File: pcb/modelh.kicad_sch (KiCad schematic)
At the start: 15 parts, among them J1 Battery Conn, J2 Conn_01x16, J3 Conn_01x12, J4 Conn_01x04, U1 nice_nano, U2 74HC595, U3 74HC595

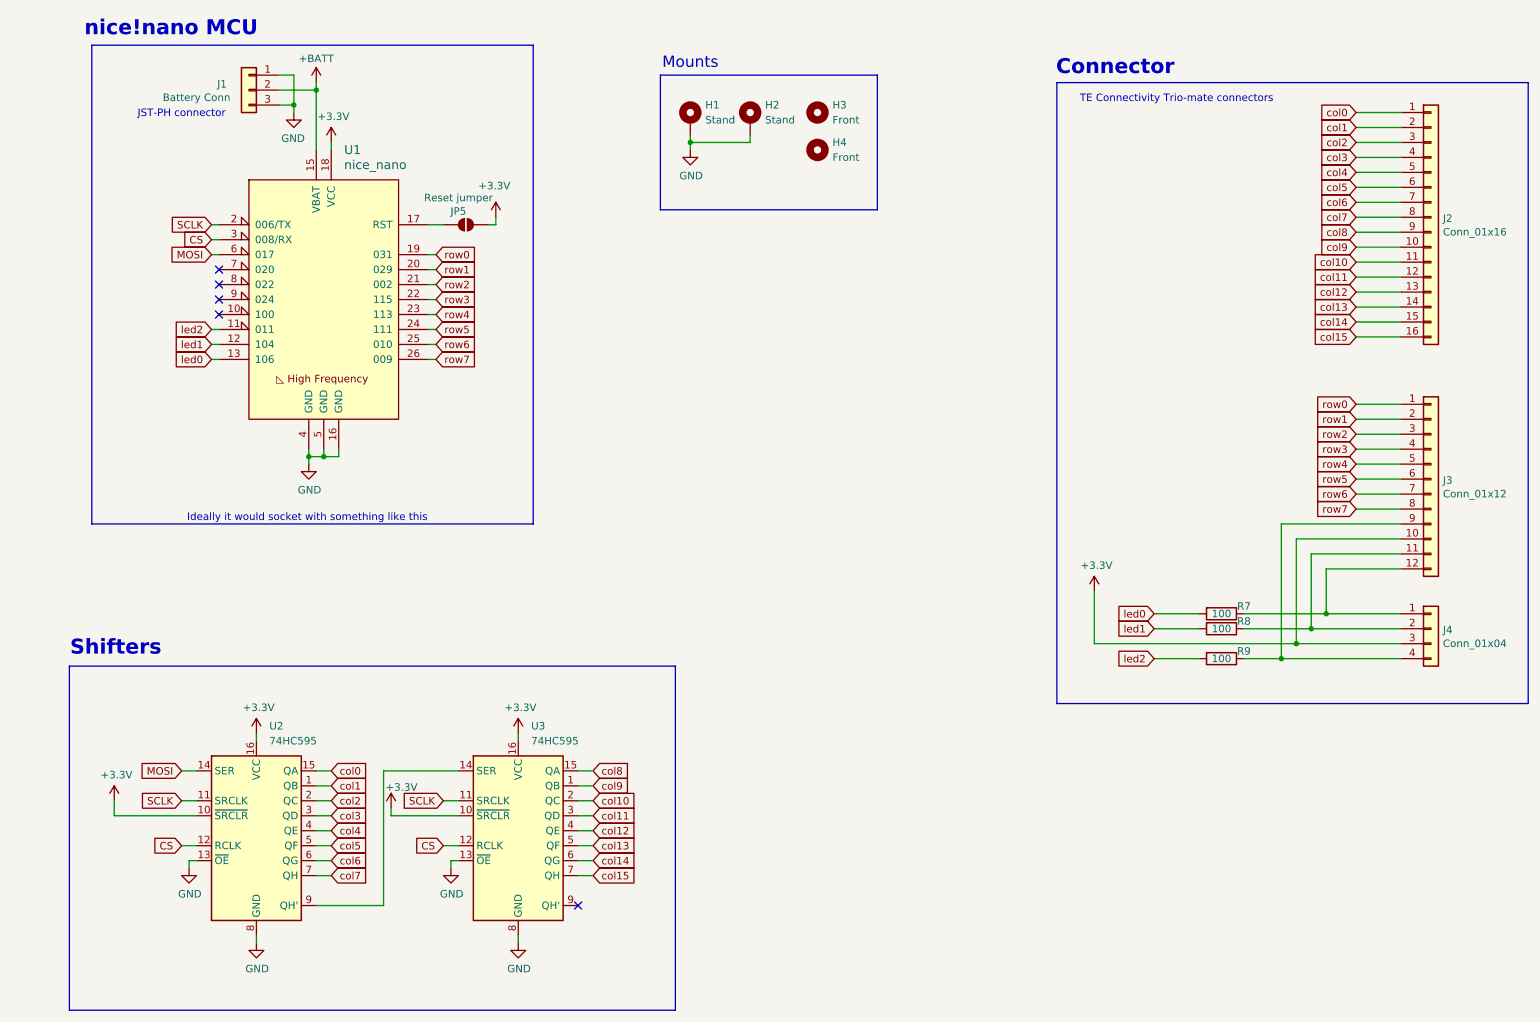
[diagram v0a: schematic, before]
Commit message: version 0.2
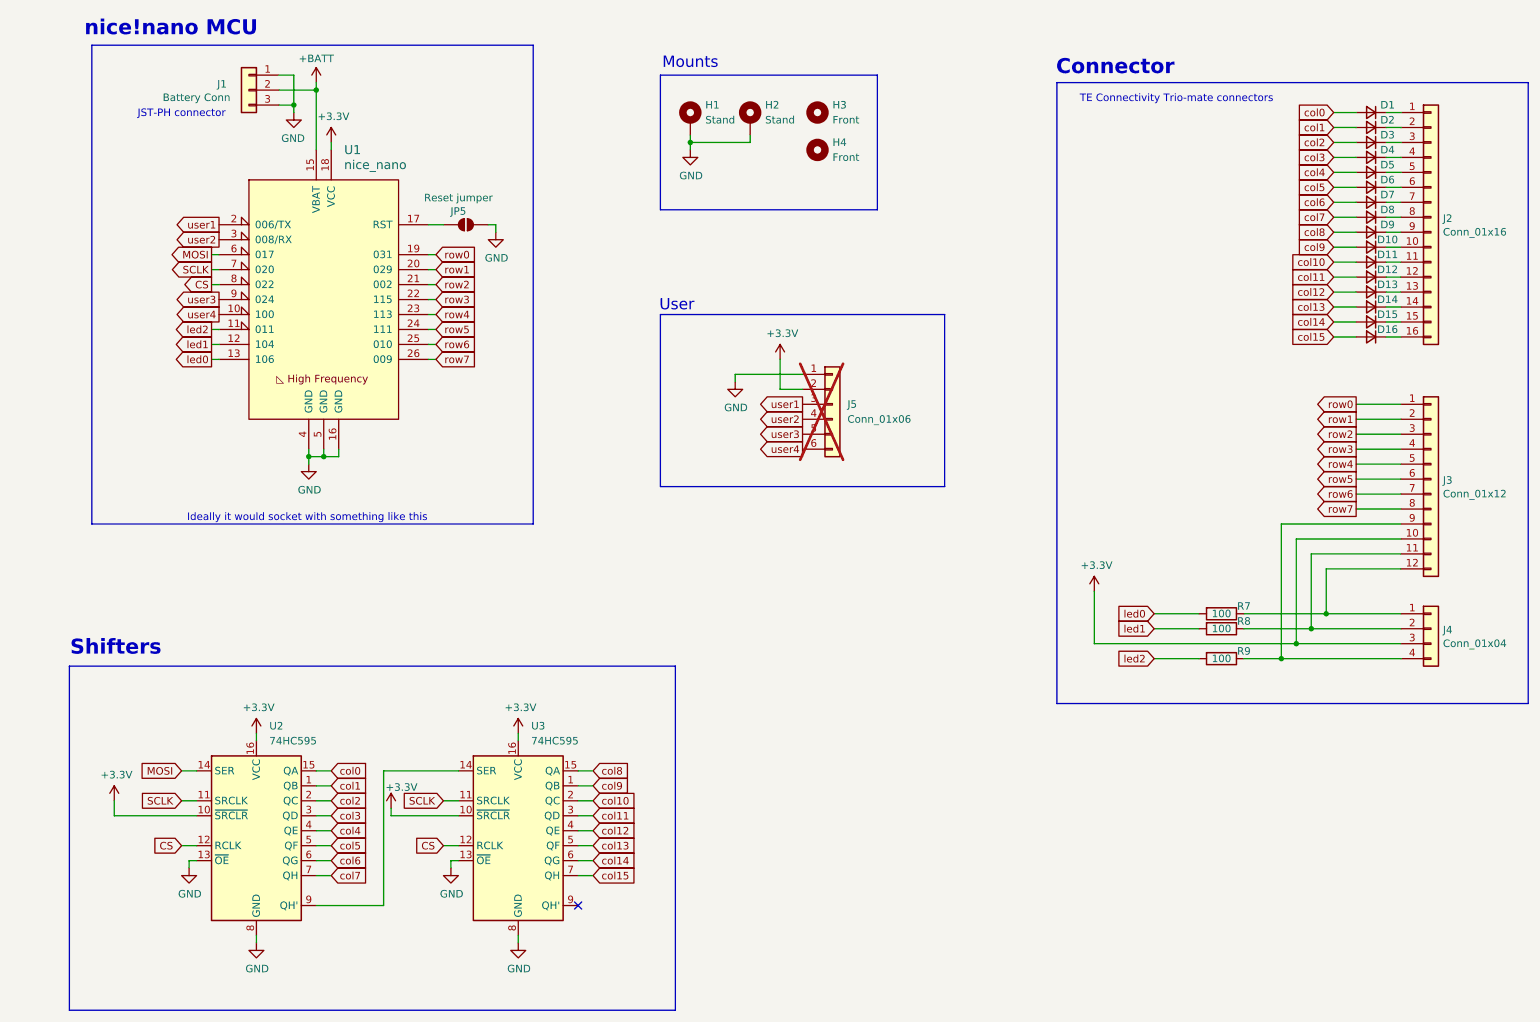
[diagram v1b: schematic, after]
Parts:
- added D1, D10, D11, D12, D13, D14, D15, D16, D2, D3, D4, D5, D6, D7, D8, D9: D_Small, Library:DO-35 smaller, symbol Device:D_Small
- added J5: Conn_01x06, Connector_PinHeader_2.54mm:PinHeader_1x06_P2.54mm_Vertical, symbol Connector_Generic:Conn_01x06
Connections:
- net +3.3V: now also J5.2 (Pin_2); no longer JP5.2 (B)
- net CS: now also U1.8 (022); no longer U1.3 (008/RX)
- net GND: now also JP5.2 (B), J5.1 (Pin_1)
- net SCLK: now also U1.7 (020); no longer U1.2 (006/TX)
- net col0: now also D1.2 (A); no longer J2.1 (Pin_1)
- net col1: now also D2.2 (A); no longer J2.2 (Pin_2)
- net col10: now also D11.2 (A); no longer J2.11 (Pin_11)
- net col11: now also D12.2 (A); no longer J2.12 (Pin_12)
- net col12: now also D13.2 (A); no longer J2.13 (Pin_13)
- net col13: now also D14.2 (A); no longer J2.14 (Pin_14)
- net col14: now also D15.2 (A); no longer J2.15 (Pin_15)
- net col15: now also D16.2 (A); no longer J2.16 (Pin_16)
- net col2: now also D3.2 (A); no longer J2.3 (Pin_3)
- net col3: now also D4.2 (A); no longer J2.4 (Pin_4)
- net col4: now also D5.2 (A); no longer J2.5 (Pin_5)
- net col5: now also D6.2 (A); no longer J2.6 (Pin_6)
- net col6: now also D7.2 (A); no longer J2.7 (Pin_7)
- net col7: now also D8.2 (A); no longer J2.8 (Pin_8)
- net col8: now also D9.2 (A); no longer J2.9 (Pin_9)
- net col9: now also D10.2 (A); no longer J2.10 (Pin_10)
- net user4: now reaches U1.10 (100)
- net user4: now also J5.6 (Pin_6)
- net user3: now reaches U1.9 (024)
- net user3: now also J5.5 (Pin_5)
- new net: D1.1 (K), J2.1 (Pin_1)
- new net: D10.1 (K), J2.10 (Pin_10)
- new net: D11.1 (K), J2.11 (Pin_11)
- new net: D12.1 (K), J2.12 (Pin_12)
- new net: D13.1 (K), J2.13 (Pin_13)
- new net: D14.1 (K), J2.14 (Pin_14)
- new net: D15.1 (K), J2.15 (Pin_15)
- new net: D16.1 (K), J2.16 (Pin_16)
- new net: D2.1 (K), J2.2 (Pin_2)
- new net: D3.1 (K), J2.3 (Pin_3)
- new net: D4.1 (K), J2.4 (Pin_4)
- new net: D5.1 (K), J2.5 (Pin_5)
- new net: D6.1 (K), J2.6 (Pin_6)
- new net: D7.1 (K), J2.7 (Pin_7)
- new net: D8.1 (K), J2.8 (Pin_8)
- new net: D9.1 (K), J2.9 (Pin_9)
- new net user1: J5.3 (Pin_3), U1.2 (006/TX)
- new net user2: J5.4 (Pin_4), U1.3 (008/RX)
- no-connect marks 5 -> 1
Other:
- note added: "User"

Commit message: Rev 0.3
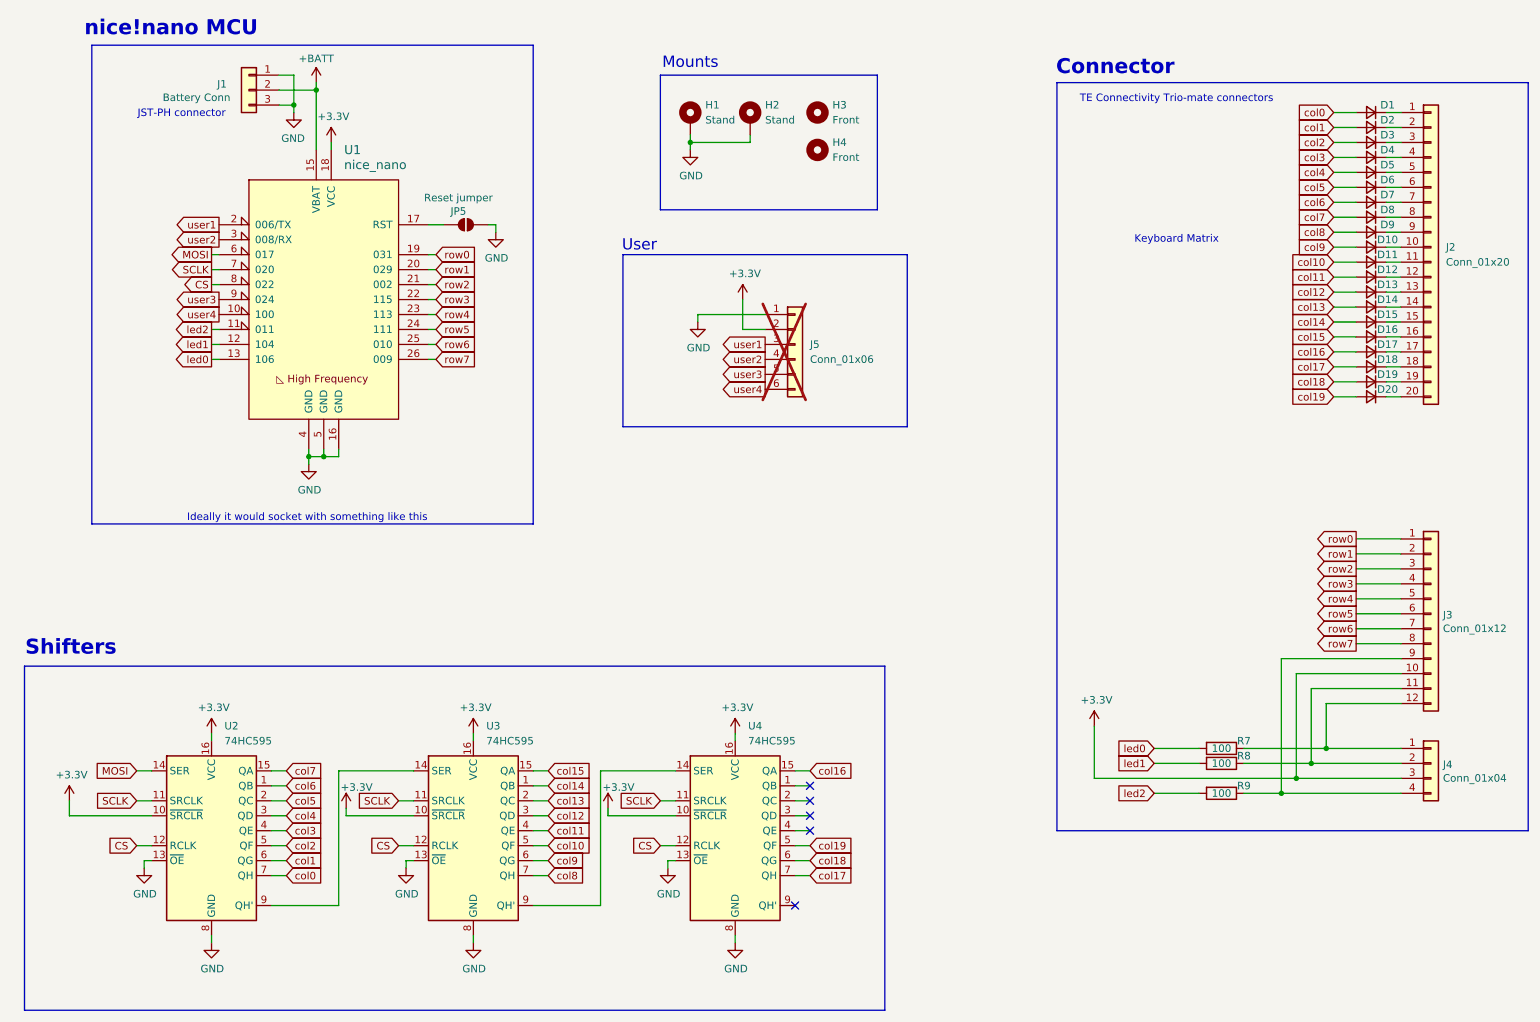
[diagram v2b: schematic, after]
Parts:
- removed J2: Conn_01x16, Library:ModelH-triomate-cols16, symbol Connector_Generic:Conn_01x16
- added D17, D18, D19, D20: D_Small, Diode_SMD:D_SOD-123F, symbol Device:D_Small
- added J2: Conn_01x20, Library:ModelH-triomate-cols20, symbol Connector_Generic:Conn_01x20
- added U4: 74HC595, Package_DIP:DIP-16_W7.62mm_Socket_LongPads, symbol 74xx:74HC595
- D1, D10, D11, D12, D13, D14, D15, D16, D2, D3, D4, D5, D6, D7, D8, D9: footprint Library:DO-35 smaller -> Diode_SMD:D_SOD-123F
- U2, U3: footprint PCM_Package_DIP_AKL:DIP-16_W7.62mm_Socket_LongPads -> Package_DIP:DIP-16_W7.62mm_Socket_LongPads
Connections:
- net +3.3V: now also U4.10 (~{SRCLR}), U4.16 (VCC)
- net CS: now also U4.12 (RCLK)
- net GND: now also U4.13 (~{OE}), U4.8 (GND)
- net SCLK: now also U4.11 (SRCLK)
- net col0: now also U2.7 (QH); no longer U2.15 (QA)
- net col1: now also U2.6 (QG); no longer U2.1 (QB)
- net col10: now also U3.5 (QF); no longer U3.2 (QC)
- net col11: now also U3.4 (QE); no longer U3.3 (QD)
- net col12: now also U3.3 (QD); no longer U3.4 (QE)
- net col13: now also U3.2 (QC); no longer U3.5 (QF)
- net col14: now also U3.1 (QB); no longer U3.6 (QG)
- net col15: now also U3.15 (QA); no longer U3.7 (QH)
- net col2: now also U2.5 (QF); no longer U2.2 (QC)
- net col3: now also U2.4 (QE); no longer U2.3 (QD)
- net col4: now also U2.3 (QD); no longer U2.4 (QE)
- net col5: now also U2.2 (QC); no longer U2.5 (QF)
- net col6: now also U2.1 (QB); no longer U2.6 (QG)
- net col7: now also U2.15 (QA); no longer U2.7 (QH)
- net col8: now also U3.7 (QH); no longer U3.15 (QA)
- net col9: now also U3.6 (QG); no longer U3.1 (QB)
- net at D1.1 (K): now also J2.1 (Pin_1)
- net at D10.1 (K): now also J2.10 (Pin_10)
- net at D11.1 (K): now also J2.11 (Pin_11)
- net at D12.1 (K): now also J2.12 (Pin_12)
- net at D13.1 (K): now also J2.13 (Pin_13)
- net at D14.1 (K): now also J2.14 (Pin_14)
- net at D15.1 (K): now also J2.15 (Pin_15)
- net at D16.1 (K): now also J2.16 (Pin_16)
- net at D2.1 (K): now also J2.2 (Pin_2)
- net at D3.1 (K): now also J2.3 (Pin_3)
- net at D4.1 (K): now also J2.4 (Pin_4)
- net at D5.1 (K): now also J2.5 (Pin_5)
- net at D6.1 (K): now also J2.6 (Pin_6)
- net at D7.1 (K): now also J2.7 (Pin_7)
- net at D8.1 (K): now also J2.8 (Pin_8)
- net at D9.1 (K): now also J2.9 (Pin_9)
- net at U3.9 (QH'): now also U4.14 (SER)
- new net: D18.1 (K), J2.18 (Pin_18)
- new net: D19.1 (K), J2.19 (Pin_19)
- new net: D20.1 (K), J2.20 (Pin_20)
- new net: D17.1 (K), J2.17 (Pin_17)
- new net col16: D17.2 (A), U4.15 (QA)
- new net col17: D18.2 (A), U4.7 (QH)
- new net col18: D19.2 (A), U4.6 (QG)
- new net col19: D20.2 (A), U4.5 (QF)
- no-connect marks 1 -> 5
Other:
- note added: "Keyboard Matrix"
- moved on the sheet: J3, J4, J5, R7, R8, R9, U2, U3
